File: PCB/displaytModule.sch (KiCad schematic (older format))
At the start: 4 parts, among them M301 DisplayModule

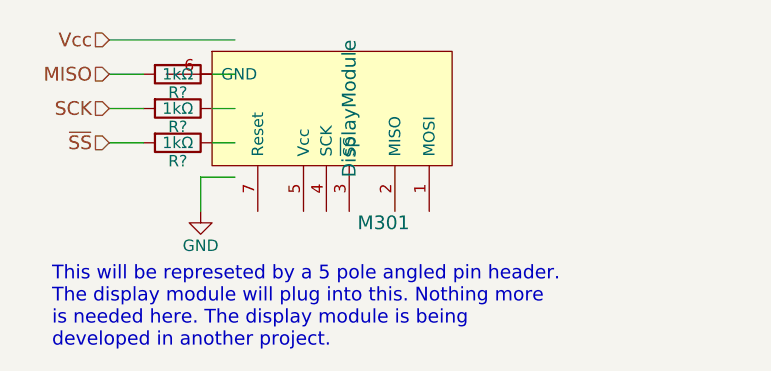
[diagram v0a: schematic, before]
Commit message: Trying out an alternative layout
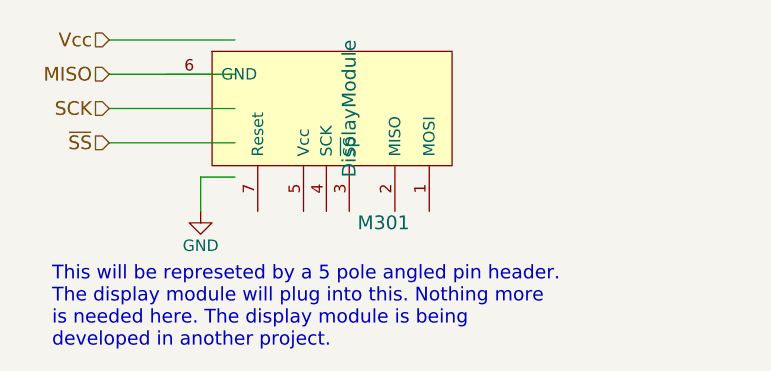
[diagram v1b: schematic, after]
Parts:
- removed R? (x3): 1kΩ, symbol R
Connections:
- wire segments 9 -> 6
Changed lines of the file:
@@
 Text Notes 2500 3000 0    60   ~ 0
 This will be represeted by a 5 pole angled pin header. \nThe display module will plug into this. Nothing more\nis needed here. The display module is being \ndeveloped in another project.
-$Comp
-L R R?
-U 1 1 55F1C62E
-P 3050 1800
-F 0 "R?" V 3130 1800 50  0000 C CNN
-F 1 "1kΩ" V 3050 1800 50  0000 C CNN
-F 2 "" V 2980 1800 30  0000 C CNN
-F 3 "" H 3050 1800 30  0000 C CNN
-	1    3050 1800
-	0    1    1    0
-$EndComp
-$Comp
-L R R?
-U 1 1 55F1C655
-P 3050 1950
-F 0 "R?" V 3130 1950 50  0000 C CNN
-F 1 "1kΩ" V 3050 1950 50  0000 C CNN
-F 2 "" V 2980 1950 30  0000 C CNN
-F 3 "" H 3050 1950 30  0000 C CNN
-	1    3050 1950
-	0    1    1    0
-$EndComp
-$Comp
-L R R?
-U 1 1 55F1C67F
-P 3050 2100
-F 0 "R?" V 3130 2100 50  0000 C CNN
-F 1 "1kΩ" V 3050 2100 50  0000 C CNN
-F 2 "" V 2980 2100 30  0000 C CNN
-F 3 "" H 3050 2100 30  0000 C CNN
-	1    3050 2100
-	0    1    1    0
-$EndComp
 Wire Wire Line
 	2750 1650 3300 1650
 Wire Wire Line
-	2750 1800 2900 1800
+	2750 1800 3300 1800
 Wire Wire Line
-	3200 1800 3300 1800
+	2750 1950 3300 1950
 Wire Wire Line
-	2750 1950 2900 1950
-Wire Wire Line
-	3200 1950 3300 1950
-Wire Wire Line
-	2750 2100 2900 2100
-Wire Wire Line
-	3200 2100 3300 2100
+	2750 2100 3300 2100
 $Comp
-L GND #PWR?
+L GND #PWR301
 U 1 1 55F1C70D
 P 3150 2400
-F 0 "#PWR?" H 3150 2150 50  0001 C CNN
+F 0 "#PWR301" H 3150 2150 50  0001 C CNN
 F 1 "GND" H 3150 2250 50  0000 C CNN
 F 2 "" H 3150 2400 60  0000 C CNN
